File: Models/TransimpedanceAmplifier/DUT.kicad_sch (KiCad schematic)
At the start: 1 part

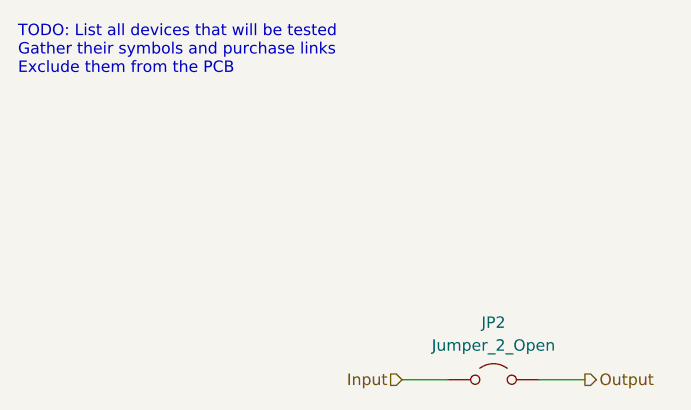
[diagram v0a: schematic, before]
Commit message: Save progress
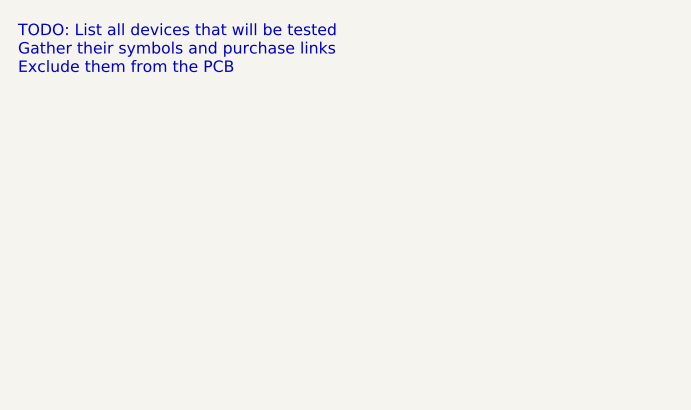
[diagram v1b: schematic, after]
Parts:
- removed JP2: Jumper_2_Open, symbol Jumper:Jumper_2_Open
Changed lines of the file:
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@@
-		)
-	)
-	(wire
-		(pts
-			(xy 144.78 91.44) (xy 149.86 91.44)
-		)
-		(stroke
-			(width 0)
-			(type default)
-		)
-	)
-	(wire
-		(pts
-			(xy 160.02 91.44) (xy 165.1 91.44)
-		)
-		(stroke
-			(width 0)
-			(type default)
-		)
-	)
-	(hierarchical_label "Output"
-		(shape output)
-		(at 165.1 91.44 0)
-		(effects
-			(font
-				(size 1.27 1.27)
-			)
-			(justify left)
-		)
-	)
-	(hierarchical_label "Input"
-		(shape input)
-		(at 144.78 91.44 180)
-		(effects
-			(font
-				(size 1.27 1.27)
-			)
-			(justify right)
-		)
-	)
-	(symbol
-		(lib_id "Jumper:Jumper_2_Open")
-		(at 154.94 91.44 0)
-		(unit 1)
-		(exclude_from_sim no)
-		(in_bom yes)
-		(on_board yes)
-		(dnp no)
-		(fields_autoplaced yes)
-		(property "Reference" "JP2"
-			(at 154.94 85.09 0)
-			(effects
-				(font
-					(size 1.27 1.27)
-				)
-			)
-		)
-		(property "Value" "Jumper_2_Open"
-			(at 154.94 87.63 0)
-			(effects
-				(font
-					(size 1.27 1.27)
-				)
-			)
-		)
-		(property "Footprint" ""
-			(at 154.94 91.44 0)
-			(effects
-				(font
-					(size 1.27 1.27)
-				)
-				(hide yes)
-			)
-		)
-		(property "Datasheet" "~"
-			(at 154.94 91.44 0)
-			(effects
-				(font
-					(size 1.27 1.27)
-				)
-				(hide yes)
-			)
-		)
-		(property "Description" "Jumper, 2-pole, open"
-			(at 154.94 91.44 0)
-			(effects
-				(font
-					(size 1.27 1.27)
-				)
-				(hide yes)
-			)
-		)
-		(pin "1"
-		)
-		(pin "2"
-		)
-		(instances
-			(project ""
-				(path "/ec9f2ae3-e40d-40eb-9760-2b611ee8efd1/dc71cb80-a5fe-4d35-8e0a-2347d37b6518"
-					(reference "JP2")
-					(unit 1)
-				)
-			)
 		)
 	)
